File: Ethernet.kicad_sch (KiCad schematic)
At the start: 7 parts, among them T401 7498111120AR, U401 TPD4EUSB30, U402 TPD4EUSB30

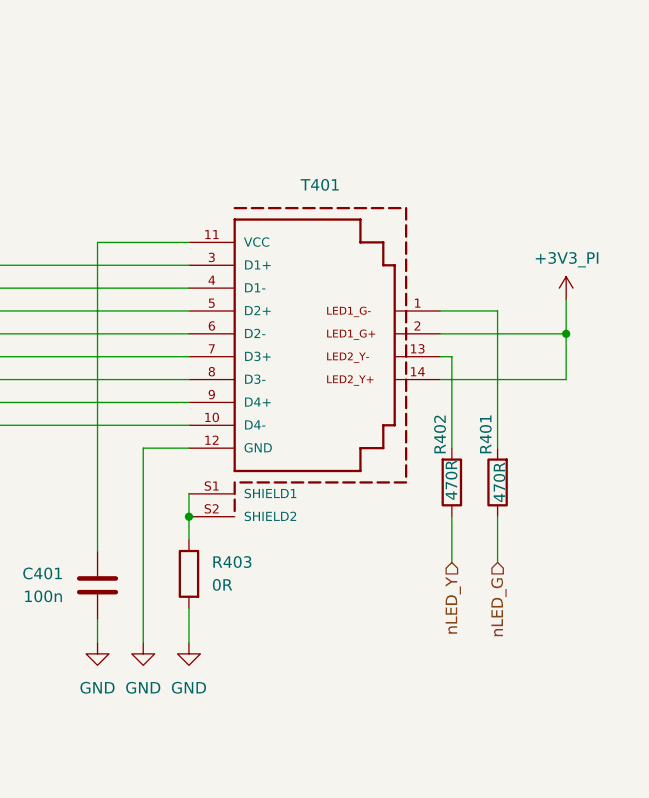
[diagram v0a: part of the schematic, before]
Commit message: eth PCB new
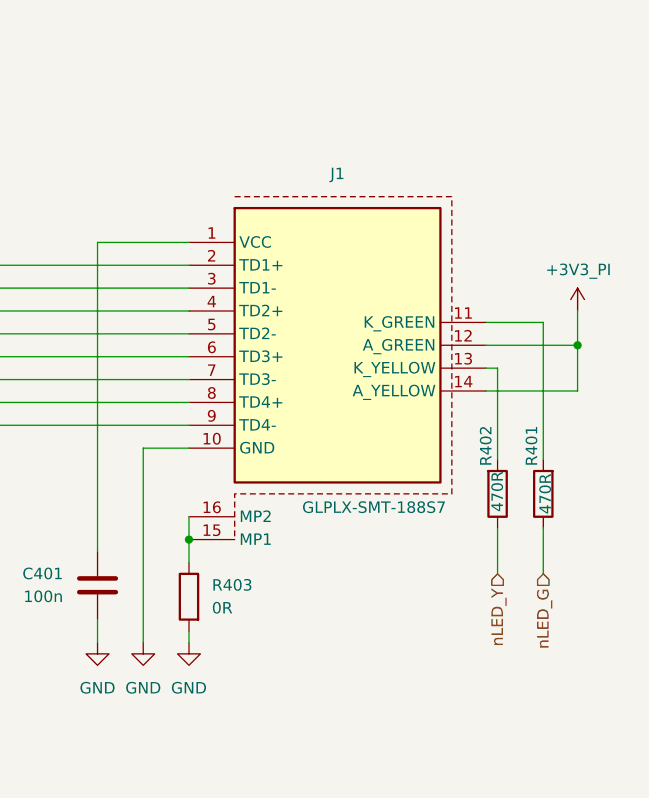
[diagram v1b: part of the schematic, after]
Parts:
- removed T401: 7498111120AR, Connector_Wuerth:7498111120AR, symbol Connector:WE-RJ45_7498111120AR
- added J1: GLPLX-SMT-188S7, GLPLXSMT188S7QQYG, symbol Samacsys:GLPLX-SMT-188S7-QQ-Y_G
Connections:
- net +3V3_PI: now also J1.12 (A_GREEN), J1.14 (A_YELLOW)
- net ETH_C.TRD0_N: now also J1.3 (TD1-)
- net ETH_C.TRD0_P: now also J1.2 (TD1+)
- net ETH_C.TRD1_N: now also J1.5 (TD2-)
- net ETH_C.TRD1_P: now also J1.4 (TD2+)
- net ETH_C.TRD2_N: now also J1.7 (TD3-)
- net ETH_C.TRD2_P: now also J1.6 (TD3+)
- net ETH_C.TRD3_N: now also J1.9 (TD4-)
- net ETH_C.TRD3_P: now also J1.8 (TD4+)
- net GND: now also J1.10 (GND)
- net at R402.2: now also J1.13 (K_YELLOW)
- net at R401.2: now also J1.11 (K_GREEN)
- net at C401.1: now also J1.1 (VCC)
- net at R403.1: now also J1.15 (MP1), J1.16 (MP2)
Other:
- moved on the sheet: R401, R402, R403

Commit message: save exit
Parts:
- J1: footprint GLPLXSMT188S7QQYG -> Samacsys:GLPLXSMT188S7QQYG
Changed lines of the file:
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@@
 			)
 		)
-		(property "Footprint" "GLPLXSMT188S7QQYG"
+		(property "Footprint" "Samacsys:GLPLXSMT188S7QQYG"
 			(at 175.26 138.1 0)
 			(effects
